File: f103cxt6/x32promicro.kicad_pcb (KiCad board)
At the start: 2 copper layers, 17.8 x 33 mm, 29 parts, among them J1 USB2.0_C_v3, J2 ProMicro-LeftPin-NoGND, J3 ProMicro-RightPin, SW1 SW_Push, SW2 SW_Push, U1 AMS1117-3.3, U2 STM32V103C8T6, Y1 32.768k, Y2 8M

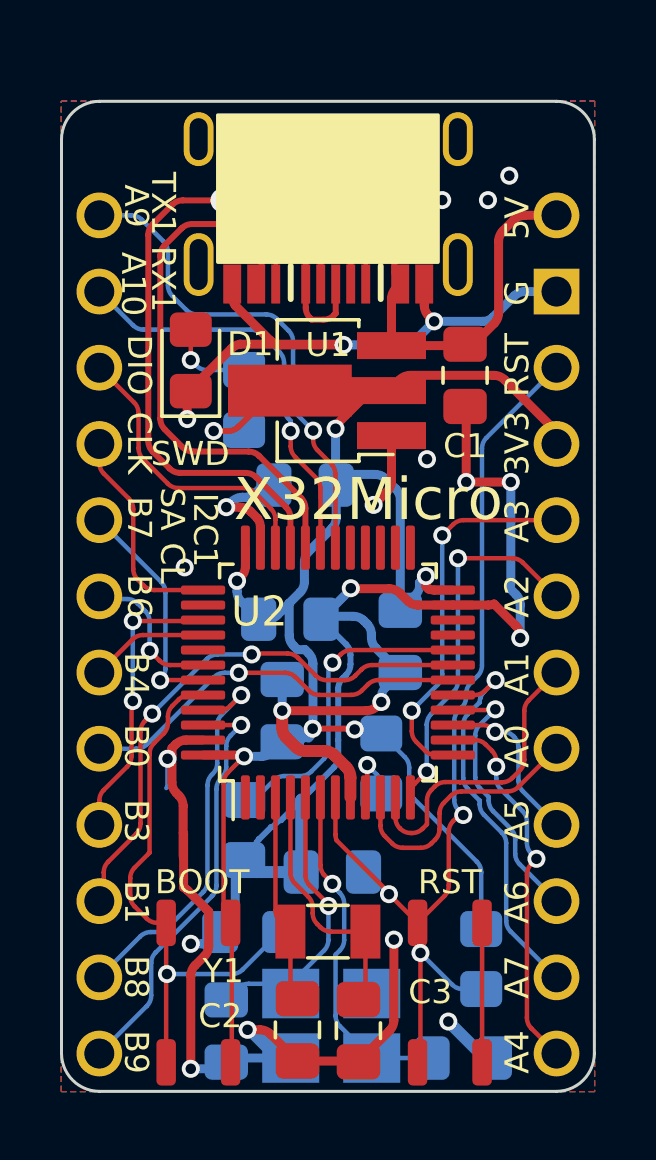
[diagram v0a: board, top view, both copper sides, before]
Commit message: v1.2.0
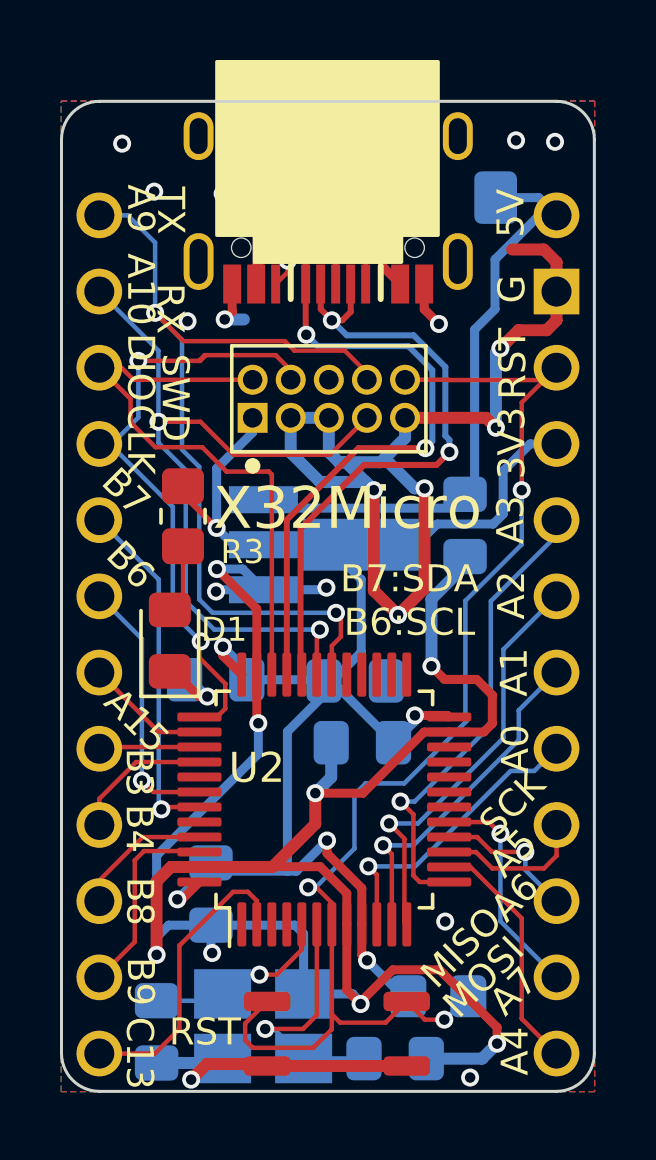
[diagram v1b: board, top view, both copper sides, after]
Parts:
- removed C10, C9: 22p, $74th:Capacitor_0805_2012
- removed C8: 100n, $74th:Capacitor_0805_2012
- removed R4: 0, $74th:Register_0805_2012
- removed R5, R6: 10k, $74th:Register_0805_2012
- removed REF**: JLCJLCJLCJLC, $74th:JLCJLCJLCJLC
- removed SW1: SW_Push, $74th:SKRPABE010
- removed Y2: 8M, $74th:Crystal_SMD_3225-4Pin_3.2x2.5mm_HandSoldering
- added F1: Polyfuse, Fuse:Fuse_1206_3216Metric_Pad1.42x1.75mm_HandSolder, B.Cu at (113.0, 103.2)
- added J4: SWD-MCU_Side-10Pin, $74th:SWD_2x05_P1.27mm, F.Cu at (106.4, 110.6)
- C1: moved to B.Cu
- C2, C3: value 12p -> 22p; moved to B.Cu
- D1: value LED -> Blue
- R3: value 200 -> 10k; moved to F.Cu
- U1: footprint Package_TO_SOT_SMD:SOT-89-3_Handsoldering -> $74th:Regulator_AMS1117_SOT-89; moved to B.Cu
- Y1: value 32.768k -> 8M; footprint $74th:Crystal_SMD_3215-2Pin_3.2x1.5mm -> $74th:Crystal_SMD_3225-4Pin_3.2x2.5mm_HandSoldering; moved to B.Cu
- moved C5 9.53 mm to (105.0, 126.4), turned to -90 degrees
- moved D1 9.37 mm to (103.6, 118.0)
- moved C4 6.74 mm to (109.8, 119.3), turned to 0 degrees
- moved C3 6.73 mm to (103.2, 131.0), turned to 90 degrees
- moved G*** 5.57 mm to (103.8, 109.2)
- moved U1 5.14 mm to (108.9, 114.8), turned to 0 degrees
- moved C1 5.00 mm to (113.5, 114.1)
- moved R3 4.51 mm to (104.1, 113.8), turned to -90 degrees
- moved U2 4.23 mm to (108.8, 123.3)
- moved SW2 4.01 mm to (109.2, 131.1), turned to 0 degrees
- moved Y1 3.82 mm to (106.7, 130.8)
- moved C6 3.61 mm to (110.0, 121.4), turned to 180 degrees
- moved C2 3.39 mm to (111.1, 131.9), turned to 180 degrees
- moved C7 2.44 mm to (105.2, 119.3), turned to 180 degrees
- moved R7 1.75 mm to (112.6, 129.8), turned to 0 degrees
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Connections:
- net 0/UART_RX renamed /0/UART_RX
- net 10/A10 renamed /10/A10
- net 14/SPI_MISO renamed /14/SPI_MISO
- net 15/SPI_SCK renamed /15/SPI_SCK
- net 16/SPI_MOSI renamed /16/SPI_MOSI
- net 18/A0 renamed /18/A0
- net 19/A1 renamed /19/A1
- net 1/UART_TX renamed /1/UART_TX
- net 20/A2 renamed /20/A2
- net 21/A3 renamed /21/A3
- net 2/I2C_SDA renamed /2/ISC_SDA
- net 3/I2C_SCL renamed /3/ISC_SCL
- net DM renamed /D-
- net DP renamed /D+
- net RST renamed /~{RESET}
- net SWCLK renamed /SWCLK
- net SWDIO renamed /SWDIO
- C2 pad 1: Net-(U1-PC14/OSC32IN) -> GND
- C2 pad 2: GND -> Net-(U2-OSC_OUT/PD1)
- C3 pad 1: Net-(U1-PC15/OSC32OUT) -> GND
- C3 pad 2: GND -> Net-(U2-OSC_IN/PD0)
- J1 pad 1: +5V -> Net-(J1-VBUS)
- J2 pad 10: 7 -> /7
- J2 pad 11: 8/A8 -> /8/A8
- J2 pad 12: 9/A9 -> /9/A9
- J2 pad 7: 4/A6 -> /4/A6
- J2 pad 8: 5 -> /5
- J2 pad 9: 6/A7 -> /6/A7
- U2 pad 18: 5 -> unconnected-(U2-PB0/ADC8-Pad18)
- U2 pad 19: 7 -> unconnected-(U2-PB1/ADC9-Pad19)
- U2 pad 2: unconnected-(U1-PC13/TAMPER_RTC-Pad2) -> /9/A9
- U2 pad 20: BOOT1 -> unconnected-(U2-BOOT1/PB2-Pad20)
- U2 pad 3: Net-(U1-PC14/OSC32IN) -> unconnected-(U2-PC14/OSC32IN-Pad3)
- U2 pad 38: unconnected-(U1-PA15-Pad38) -> /4/A6
- U2 pad 39: 6/A7 -> /5
- U2 pad 4: Net-(U1-PC15/OSC32OUT) -> unconnected-(U2-PC15/OSC32OUT-Pad4)
- U2 pad 40: 4/A6 -> /6/A7
- U2 pad 44: BOOT0 -> unconnected-(U2-BOOT0-Pad44)
- U2 pad 45: 8/A8 -> /7
- U2 pad 46: 9/A9 -> /8/A8
- U2 pad 5: Net-(U1-OSC_IN/PD0) -> Net-(U2-OSC_IN/PD0)
- U2 pad 6: Net-(U1-OSC_OUT/PD1) -> Net-(U2-OSC_OUT/PD1)
- U2 pad 9: Net-(U1-VDDA) -> +3V3
- Y1 pad 1: Net-(U1-PC15/OSC32OUT) -> Net-(U2-OSC_IN/PD0)
- Y1 pad 2: Net-(U1-PC14/OSC32IN) -> GND
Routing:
- net BOOT0: track 18.6 -> 0.00 mm, vias 1 -> 0
- net 7: track 18.2 -> 0.00 mm, vias 2 -> 0
- net /SWCLK: track 7.28 -> 21.3 mm, vias 0 -> 2
- net 9/A9: track 14.0 -> 0.00 mm, vias 1 -> 0
- net /1/UART_TX: track 16.5 -> 30.0 mm, vias 1 -> 2
- net 5: track 13.2 -> 0.00 mm, vias 1 -> 0
- net 8/A8: track 13.0 -> 0.00 mm, vias 1 -> 0
- net /0/UART_RX: track 13.8 -> 25.8 mm, vias 1 -> 2
- net Net-(U1-OSC_OUT/PD1): track 11.6 -> 0.00 mm, vias 1 -> 0
- net BOOT1: track 10.3 -> 0.00 mm, vias 1 -> 0
- net /9/A9: track 0.00 -> 10.0 mm
- net /SWDIO: track 9.83 -> 19.6 mm
- net 6/A7: track 9.59 -> 0.00 mm, vias 2 -> 0
- net GND: track 113.6 -> 123.1 mm, vias 22 -> 28
- net Net-(U1-OSC_IN/PD0): track 9.33 -> 0.00 mm, vias 1 -> 0
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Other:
- board text added: "A15"
- board text added: "B7:SDA B6:SCL"
- board text added: "C13"
- board text added: "MISO"
- board text added: "MOSI"
- board text added: "RX"
- board text added: "SCK"
- board text added: "TX"
- board text added: "v1.2.0"
- board text removed: "B0"
- board text removed: "B1"
- board text removed: "BOOT"
- board text removed: "CL"
- board text removed: "I2C1"
- board text removed: "SA"
- board text removed: "TX1 RX1"
- board text removed: "v1.1.2"
- board text removed: ""
